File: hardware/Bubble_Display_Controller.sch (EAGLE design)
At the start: 37 parts, among them J1 ICSP, Q1 BSS84, Q10 IRFML8244, Q11 IRFML8244, Q12 IRFML8244, Q13 IRFML8244, Q14 IRFML8244, Q15 IRFML8244, Q16 IRFML8244, Q2 BSS84, Q3 BSS84, Q4 BSS84, Q5 BSS84, Q6 BSS84, Q7 BSS84, Q8 BSS84, Q9 IRFML8244, U4 ATMEGA328, Y1 16MHz

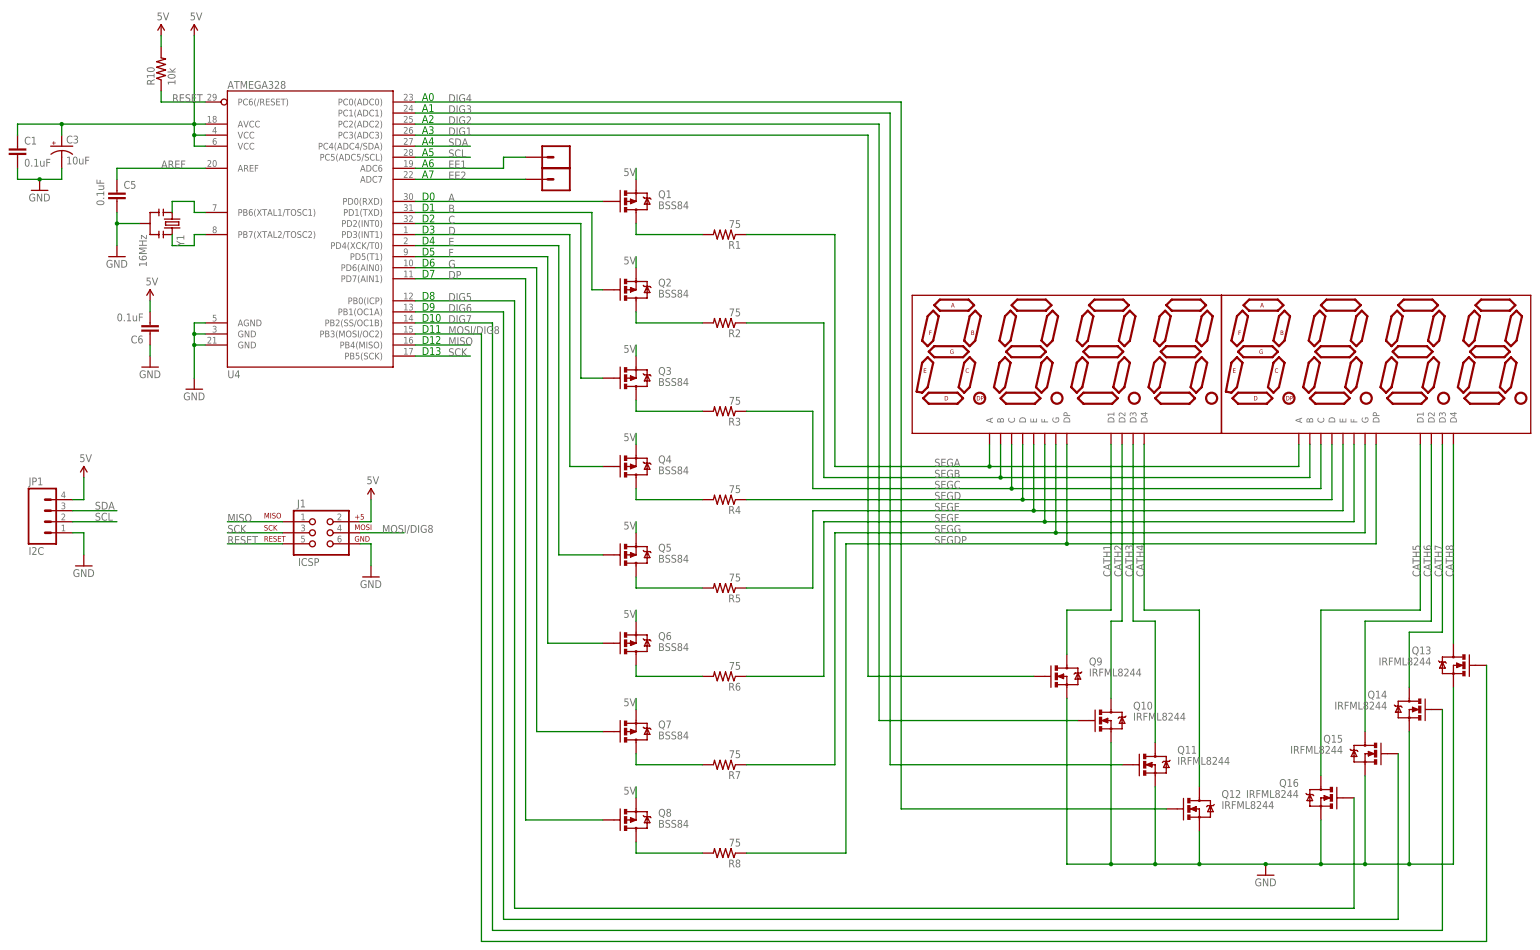
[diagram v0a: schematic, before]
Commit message: New HW version started. Bringing FW forward.
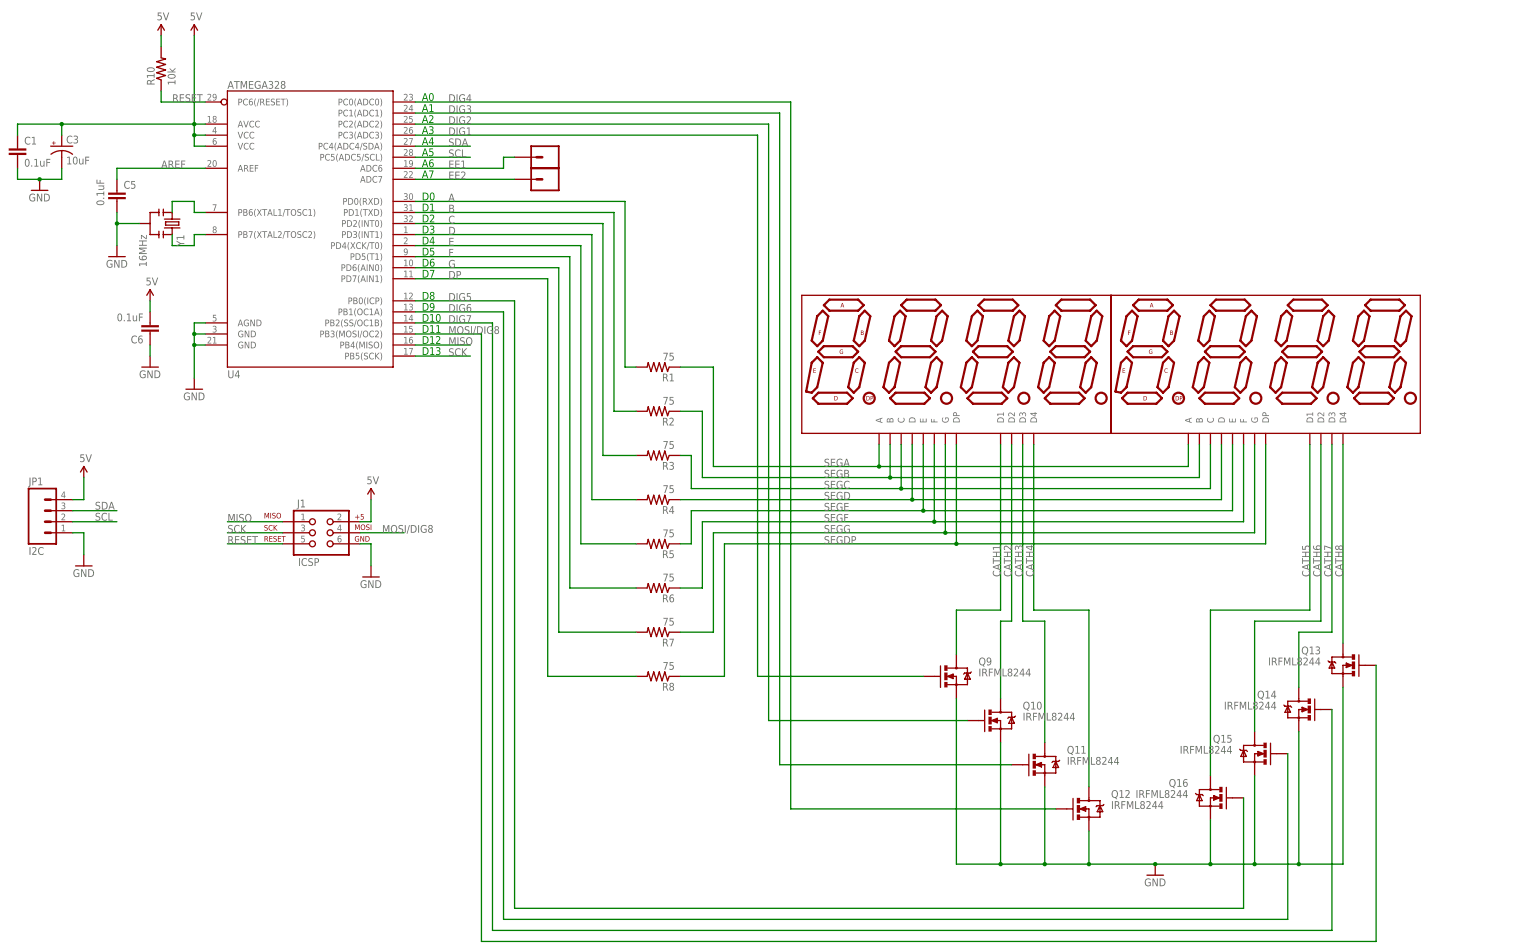
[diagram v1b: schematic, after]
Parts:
- removed Q1, Q2, Q3, Q4, Q5, Q6, Q7, Q8: BSS84, SparkFun-DiscreteSemi:MOSFET-PCHANNELSMD
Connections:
- removed net N$23: Q5.D, R5.2
- removed net N$25: Q1.D, R1.2
- removed net N$27: Q6.D, R6.2
- removed net N$28: Q2.D, R2.2
- removed net N$30: Q3.D, R3.2
- removed net N$32: Q4.D, R4.2
- removed net N$33: Q7.D, R7.2
- removed net N$34: Q8.D, R8.2
- net 5V: no longer Q1.S, Q2.S, Q3.S, Q4.S, Q5.S, Q6.S, Q7.S, Q8.S
- net A: now also R1.2; no longer Q1.G
- net B: now also R2.2; no longer Q2.G
- net C: now also R3.2; no longer Q3.G
- net D: now also R4.2; no longer Q4.G
- net DP: now also R8.2; no longer Q8.G
- net E: now also R5.2; no longer Q5.G
- net F: now also R6.2; no longer Q6.G
- net G: now also R7.2; no longer Q7.G
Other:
- moved on the sheet: Q10, Q11, Q12, Q13, Q14, Q15, Q16, Q9, R1, R2, R3, R4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
